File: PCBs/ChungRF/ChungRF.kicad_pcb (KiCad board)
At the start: 4 copper layers, 28.4 x 53.4 mm, 15 parts, among them J1 Conn_Coaxial, J2 Conn_01x09_Socket, U1 E22-900M30S

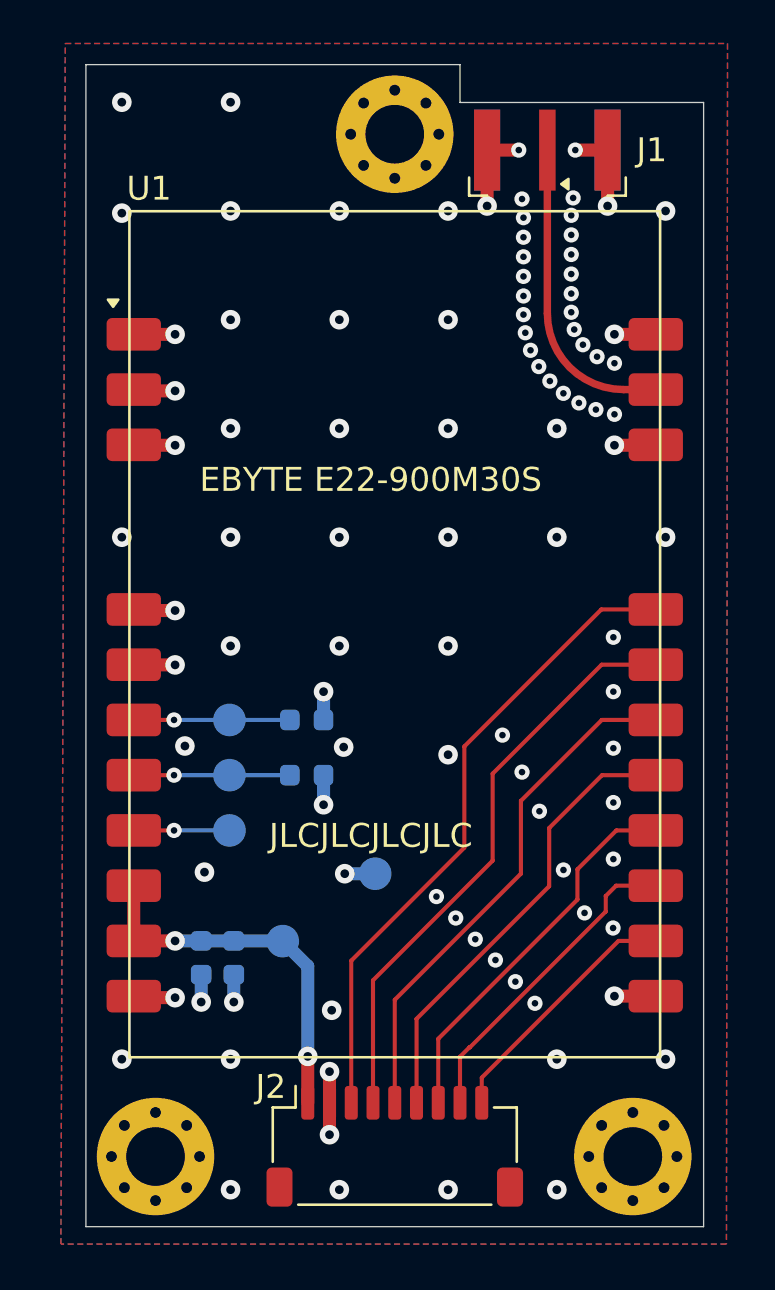
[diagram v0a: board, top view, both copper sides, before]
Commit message: ChungRF R2
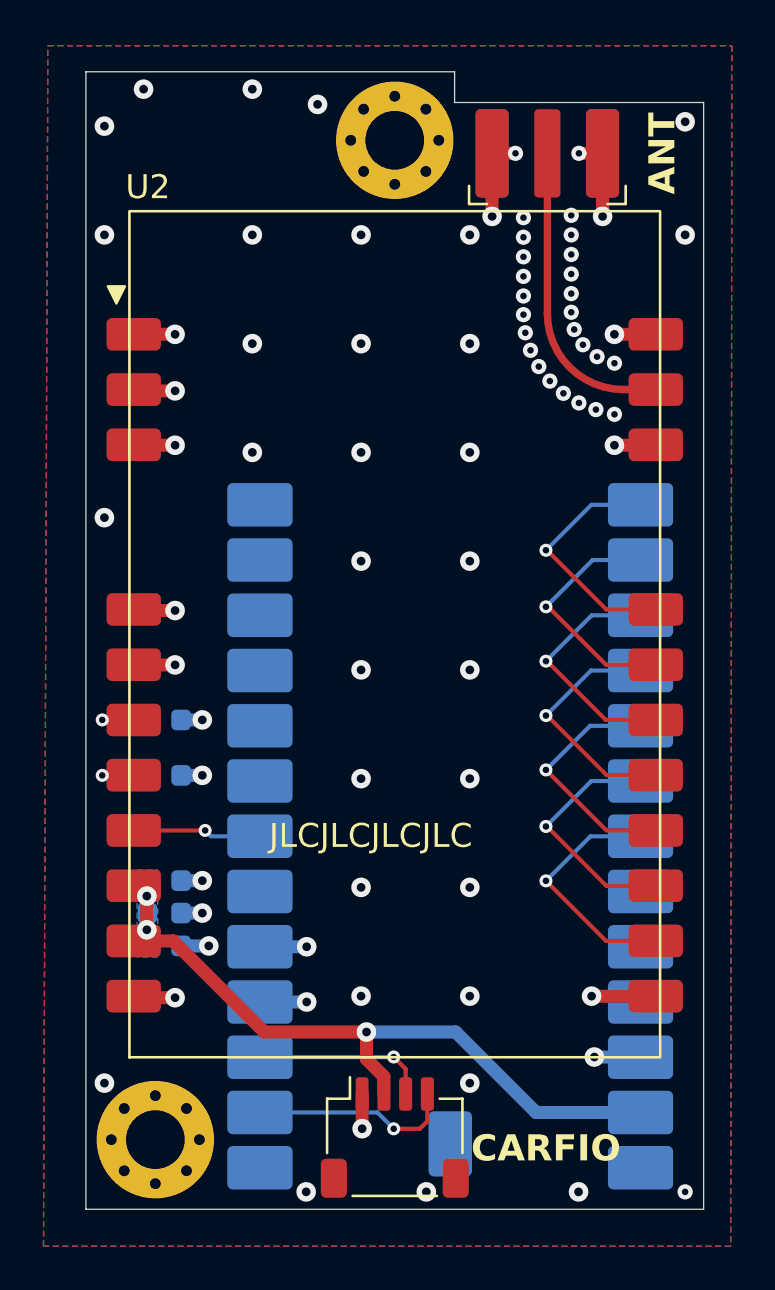
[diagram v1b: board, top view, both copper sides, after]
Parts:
- removed H3: MountingHole, MountingHole:MountingHole_2.7mm_M2.5_Pad_Via
- removed TP1: VCC, TestPoint:TestPoint_Pad_D1.5mm
- removed TP2: GND, TestPoint:TestPoint_Pad_D1.5mm
- removed TP3: RXEN, TestPoint:TestPoint_Pad_D1.5mm
- removed TP4: TXEN, TestPoint:TestPoint_Pad_D1.5mm
- removed TP5: DIO2, TestPoint:TestPoint_Pad_D1.5mm
- added C3: 10uF, Capacitor_SMD:C_0603_1608Metric, B.Cu at (154.9, 98.7)
- added U1: KB2040, besser_footprints:Adafuit-KB2040-SMD, B.Cu at (168.1, 96.7)
- H1, H2: value MountingHole -> 2.7mm_M2.5_Pad_Via
- J1: value Conn_Coaxial -> JST-SM04B-SRSS; footprint besser_footprints:CON-SMA-EDGE-S -> besser_footprints:JST_SH_SM04B-SRSS-TB_1x04-1MP_P1.00mm_Horizontal
- J2: value Conn_01x09_Socket -> Conn_Coaxial; footprint Connector_JST:JST_SH_SM09B-SRSS-TB_1x09-1MP_P1.00mm_Horizontal -> besser_footprints:CONSMA003.062
- R1, R2: value 100k -> 10k
- moved H1 48.0 mm to (165.5, 64.7), turned to 0 degrees
- moved J2 46.2 mm to (172.6, 65.2)
- moved J1 45.9 mm to (165.5, 110.5)
- moved H2 22.0 mm to (154.5, 110.6), turned to 0 degrees
- moved R2 6.55 mm to (154.9, 93.8)
- moved R1 6.55 mm to (154.9, 91.3)
- moved C2 3.80 mm to (154.9, 100.2), turned to 0 degrees
- moved C1 1.78 mm to (154.9, 101.7), turned to 0 degrees
- renumbered U1 to U2
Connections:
- C1 pad 1: VCC -> VBUS
- C2 pad 1: VCC -> VBUS
- J1 pad 1: /RF_ANT -> GND
- J1 pad 2: GND -> VBUS
- J2 pad 1: VCC -> /RF_ANT
- U2 pad 10: VCC -> VBUS
- U2 pad 9: VCC -> VBUS
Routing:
- net VBUS: track 0.00 -> 31.3 mm, vias 0 -> 3
- net /NSS: track 29.9 -> 11.9 mm, vias 0 -> 1
- net VCC: track 17.2 -> 0.00 mm, vias 2 -> 0
- net /SCK: track 27.0 -> 11.8 mm, vias 0 -> 1
- net /MOSI: track 24.0 -> 11.4 mm, vias 0 -> 1
- net /MISO: track 21.1 -> 11.4 mm, vias 0 -> 1
- net /CARFIO_MOSI: track 0.00 -> 9.41 mm, vias 0 -> 1
- net /CARFIO_MISO: track 0.00 -> 8.08 mm, vias 0 -> 1
- net /NRST: track 17.7 -> 11.5 mm, vias 0 -> 1
- net GND: track 34.6 -> 39.3 mm, vias 99 -> 79
- net /RXEN: track 7.18 -> 3.52 mm
- net /BUSY: track 14.8 -> 11.4 mm, vias 0 -> 1
- net /TXEN: track 7.18 -> 4.88 mm
- net /DIO2: track 4.40 -> 5.91 mm
- net /DIO1: track 11.8 -> 11.4 mm, vias 0 -> 1
- added copper zone on B.Cu, net VBUS
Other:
- board size 28.4 x 53.4 mm -> 28.4 x 52.3 mm
- board text added: "ANT"
- board text added: "CARFIO"
- board text added: "R2 6-2024"
- board text removed: "Chungus Aerospace"
- board text removed: "DIO2"
- board text removed: "EBYTE E22-900M30S"
- board text removed: "GND"
- board text removed: "R2 5-2024"
- board text removed: "RXEN"
- board text removed: "TXEN"
- board text removed: "VCC"
